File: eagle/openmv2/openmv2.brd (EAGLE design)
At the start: 43.2 x 54.6 mm, 82 parts, among them J3 CON_HEADER_1X03, J4 CON_HEADER_1X03, Q1 MOSFET, U1 TPS2114APW, U10 IS42S81600E-7TL, U2 USD-47571, U3 BEAD, U4 TPS768, U5 BEAD, U6 BEAD, U7 STM32F429, U8 VREG_25, U9 OV2640, X1 USB-MICROB

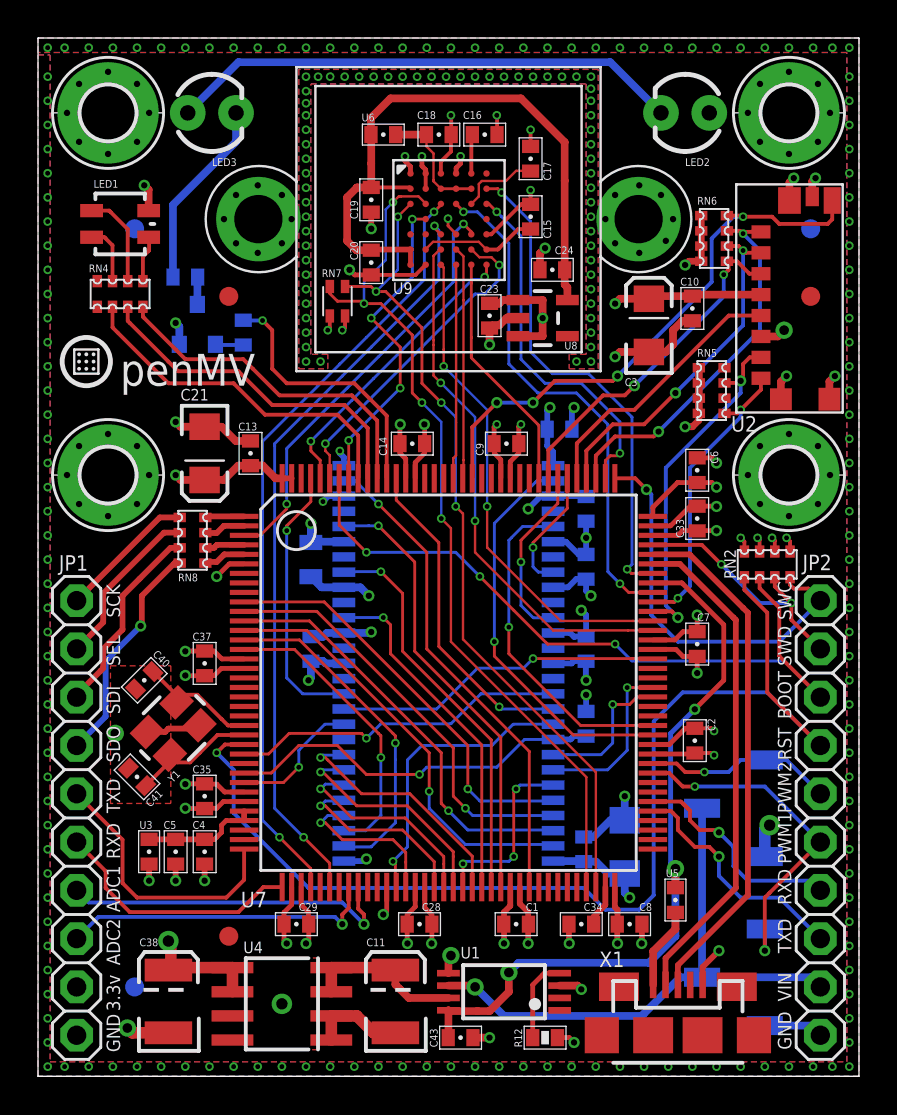
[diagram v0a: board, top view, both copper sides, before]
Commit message: Rename Eagle files
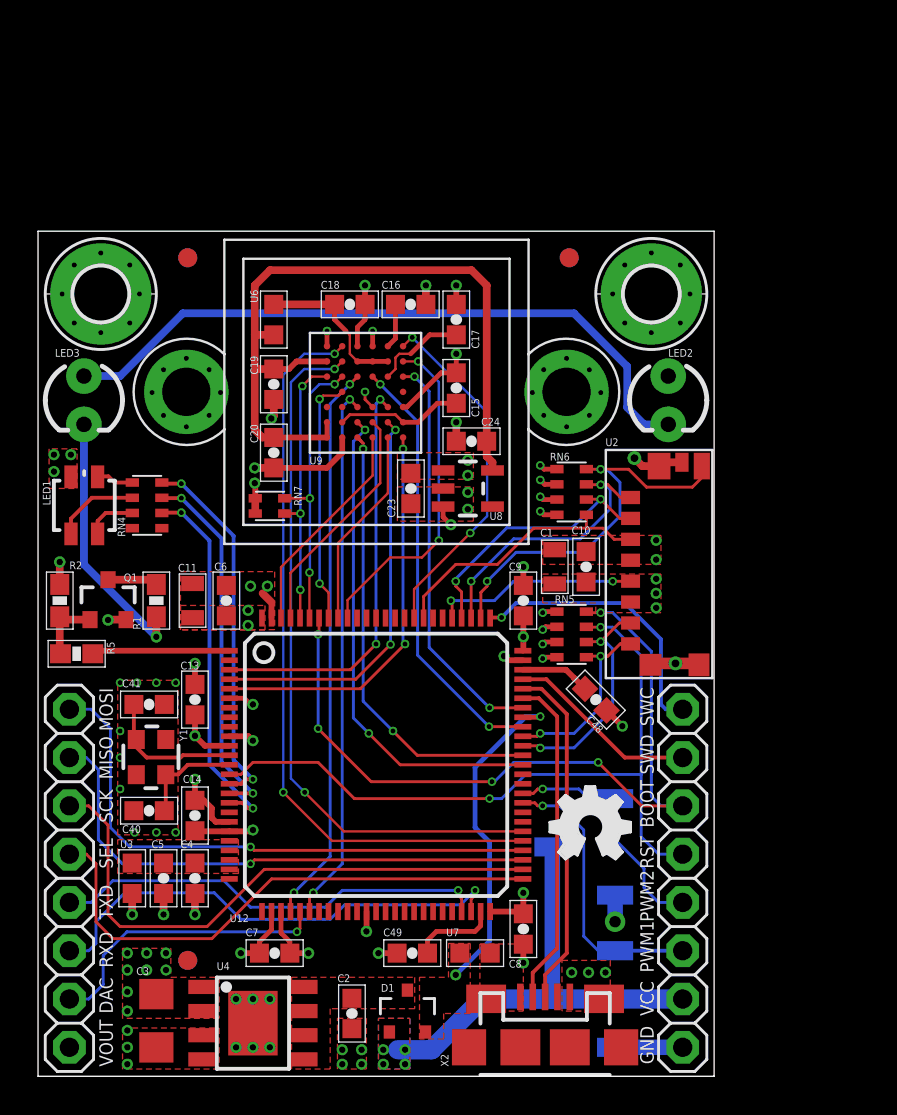
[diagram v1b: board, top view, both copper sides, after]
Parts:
- removed C12, C21: 100uF, sfe:EIA3216
- removed C25, C26, C27, C28, C29, C31, C32, C35, C36, C37, C43: 0.1uF, sfe:0402-CAP
- removed C30: 10uF, sfe:0805
- removed C33, C34: 2.2uF, sfe:0402-CAP
- removed C38: 100uF, sfe:EIA3528
- removed H1, H8: MOUNT-PAD-ROUND2.8, holes:2,8-PAD
- removed R12: 1K, sfe:0402-RES
- removed R4: 10ohm, iofault:0402-RES
- removed RN2, RN8: (no value), resistor-dil:CAT16
- removed U$1: LENSMOUNT, omnivision:LENSMOUNT
- removed U$14, U$15, U$16, U$17, U$19, U$20: FIDUCIAL, adafruit:FIDUCIAL_1MM
- removed U10: IS42S81600E-7TL, mux:TSOPII-54
- removed U5: BEAD, heka:0402-CAP
- removed X1: USB-MICROB, sfe:USB-MICROB
- added C48, C49: 2.2uF, sfe:0603-CAP
- added D1: BAT54C, diode:SOT23
- added JP3, JP4: (no value), pinhead:1X08
- added JP5, JP6, JP7, JP8: FIDUCIAL1X2, sfe:FIDUCIAL-1X2
- added R2: 10k, sfe:0603-RES
- added U$3: (no value), openmv:OMV-LOGO
- added U12: STM32F427-LQFP100, mux:LQFP100
- added X2: USB-MICROB, sfe:USB-MICROB
- C1: value 0.1uF -> 22uF; device sfe:0402-CAP -> sfe:0805
- C10, C13, C14, C15, C16, C17, C18, C19, C20, C4, C5, C6, C7, C8, C9: device sfe:0402-CAP -> sfe:0603-CAP
- C11: value 100uF -> 22uF; device sfe:EIA3528 -> sfe:0805
- C2: value 0.1uF -> 4.7uF; device sfe:0402-CAP -> sfe:0603-CAP
- C23, C24: value 10uF -> 4.7uF; device sfe:0402-CAP -> sfe:0603-CAP
- C3: device sfe:EIA3216 -> sfe:1206
- C40, C41: value 18pF -> 12pF; device sfe:0402-CAP -> sfe:0603-CAP
- JP1, JP2: value (none) -> FIDUCIAL1X2; device pinhead:1X10 -> sfe:FIDUCIAL-1X2
- LOGO1: value OSHW_LOGO_FILLX0200-NT -> OSHW_LOGO_FILLX0150-NT; device iofault:OSHW_FILLX200_NOTEXT -> iofault:OSHW_FILLX150_NOTEXT
- R1: value 10K -> 10ohm; device sfe:0402-RES -> sfe:0603-RES
- R5: device sfe:0402-RES -> sfe:0603-RES
- RN4: value (none) -> 220R; device resistor-dil:CAT16 -> resistor-dil:EXBV8V
- RN5, RN6: value (none) -> 10K; device resistor-dil:CAT16 -> resistor-dil:EXBV8V
- RN7: value (none) -> 10K
- U1: value TPS2114APW -> LENSMOUNT20MM; device mux:TSSOP8 -> omnivision:LENSMOUNT-20MM
- U3, U6: value BEAD -> (none); device heka:0402-CAP -> sfe:0603
- U4: value TPS768 -> BD33IA; device mux:SOIC8 -> mux:HTSOP-J8
- U7: value STM32F429 -> (none); device stm32:LQFP144 -> sfe:0603
- U8: value VREG_25 -> VREG_28
- Y1: device mux:CRYSTAL3.2X2.5 -> mux:CRYSTAL-2.5X2.0
- moved C3 44.8 mm to (6.22, 2.92), turned to 270 degrees
- moved H2 37.4 mm to (3.30, 41.1)
- moved JP2 34.1 mm to (7.87, 6.10), flipped to the bottom, turned to 0 degrees
- moved U1 32.3 mm to (17.8, 36.0), turned to 0 degrees
- moved H6 30.1 mm to (32.3, 41.1)
- moved C7 27.5 mm to (12.4, 6.48), turned to 180 degrees
- moved C6 25.7 mm to (9.91, 25.0)
- moved C11 23.6 mm to (8.13, 25.0), turned to 270 degrees
- moved R1 23.5 mm to (6.22, 25.0), flipped to the top
- moved C2 23.0 mm to (16.5, 3.30)
- moved C14 22.7 mm to (8.26, 13.7), turned to 270 degrees
- moved R5 19.0 mm to (2.03, 22.2), flipped to the top, turned to 180 degrees
- moved C1 18.9 mm to (27.2, 26.8), turned to 270 degrees
- moved LOGO1 16.7 mm to (26.9, 11.4), flipped to the top
- moved LED3 16.5 mm to (2.41, 35.6), turned to 270 degrees
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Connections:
- removed net ADC12_IN14: JP1.8, U7.44
- removed net ADC12_IN15: JP1.7, U7.45
- removed net ADC12_IN5: U7.41
- removed net DCMI_SCL: RN7.2, U7.69, U9.C2
- removed net DCMI_SDA: RN7.1, U7.70, U9.C1
- removed net DRAM_A0: U10.23, U7.10
- removed net DRAM_A1: U10.24, U7.11
- removed net DRAM_A10: U10.22, U7.56
- removed net DRAM_A11: U10.35, U7.57
- removed net DRAM_A2: U10.25, U7.12
- removed net DRAM_A3: U10.26, U7.13
- removed net DRAM_A4: U10.29, U7.14
- removed net DRAM_A5: U10.30, U7.15
- removed net DRAM_A6: U10.31, U7.50
- removed net DRAM_A7: U10.32, U7.53
- removed net DRAM_A8: U10.33, U7.54
- removed net DRAM_A9: U10.34, U7.55
- removed net DRAM_BA0: U10.20, U7.89
- removed net DRAM_BA1: U10.21, U7.90
- removed net DRAM_CAS: U10.17, U7.132
- removed net DRAM_CLK: U10.38, U7.93
- removed net DRAM_CLKE: U10.37, U7.29
- removed net DRAM_CS: R1.2, U10.19, U7.28
- removed net DRAM_D0: U10.2, U7.85
- removed net DRAM_D1: U10.5, U7.86
- removed net DRAM_D2: U10.8, U7.114
- removed net DRAM_D3: U10.11, U7.115
- removed net DRAM_D4: U10.44, U7.58
- removed net DRAM_D5: U10.47, U7.59
- removed net DRAM_D6: U10.50, U7.60
- removed net DRAM_D7: U10.53, U7.63
- removed net DRAM_DQM: U10.39, U7.141
- removed net DRAM_RAS: U10.18, U7.49
- removed net DRAM_WE: U10.16, U7.26
- removed net FS_DN: U7.103, X1.D-
- removed net N$15: U7.128
- removed net N$17: U7.92
- removed net N$18: U7.18
- removed net N$19: U7.91
- removed net N$20: JP1.1, RN8.1
- removed net N$21: JP1.2, RN8.2
- removed net N$22: U5.1, X1.VBUS
- removed net N$23: JP1.3, RN8.3
- removed net N$24: JP1.4, RN8.4
- removed net N$25: U7.122
- removed net N$26: R12.2, U1.4
- removed net N$27: U7.19
- removed net N$28: U7.20
- removed net SPI4_MISO: RN8.6, U7.4
- removed net SPI4_MOSI: RN8.5, U7.5
- removed net SPI4_NSS: RN8.7, U7.2
- removed net SPI4_SCK: RN8.8, U7.1
- removed net TIM12_CH1: U7.75
- removed net TIM12_CH2: U7.76
- removed net USART2_RX: JP1.6, U7.37
- removed net USART2_TX: JP1.5, U7.36
- removed net USART3_RX: JP2.7, U7.78
- removed net USART3_TX: JP2.8, U7.77
- removed net VBAT: J3.2, J4.2, JP2.9, U1.6
- new net DAC: JP4.7, U12.30
- new net EXPST: U12.55, U9.A2
- new net FREX: U12.56, U9.B2
- new net FS_DM: U12.70, X2.D-
- new net I2C1_SCL: RN7.2, U12.95, U9.C2
- new net I2C1_SDA: RN7.1, U12.96, U9.C1
- new net I2C2_SCL: JP4.5, U12.47
- new net I2C2_SDA: JP4.6, U12.48
- new net RAW: D1.1, J3.2, J4.2, JP3.7
- new net SPI2_MISO: JP4.2, U12.53
- new net SPI2_MOSI: JP4.1, U12.54
- new net SPI2_NSS: JP4.4, U12.51
- new net SPI2_SCLK: JP4.3, U12.52
- new net STROBE: U12.84, U9.A6
- net BOOT0: now also JP3.3, RN5.8, U12.94; no longer JP2.3, RN2.6, U7.138
- net DCMI_CLK: now also U12.67; no longer U7.100
- net DCMI_D0: now also U12.63; no longer U7.96
- net DCMI_D1: now also U12.64; no longer U7.97
- net DCMI_D2: now also U12.97; no longer U7.125
- net DCMI_D3: now also U12.98; no longer U7.126
- net DCMI_D4: now also U12.3; no longer U7.3
- net DCMI_D5: now also U12.92; no longer U7.117
- net DCMI_D6: now also U12.4; no longer U7.139
- net DCMI_D7: now also U12.5; no longer U7.140
- net DCMI_HSYNC: now also U12.29; no longer U7.40
- net DCMI_PCLK: now also U12.31; no longer U7.42
- net DCMI_PWDN: now also U12.91; no longer U7.102
- net DCMI_RST: now also U12.69; no longer U7.110
- net DCMI_VSYNC: now also U12.93; no longer U7.137
- net FS_DP: now also U12.71, X2.D+; no longer U7.104, X1.D+
- net GND: now also C11.1, C3.2, C48.2, C49.2, JP3.8, R2.1, RN5.1, U12.10, U12.20, U12.27, U12.37, U12.74, U12.99, U4.3, U4.P$1, X2.GND; no longer C11.C, C12.C, C21.C, C25.2, C26.2, C27.2, C28.1, C29.2, C3.C, C30.2, C31.2, C32.2, C33.2, C34.2, C35.2, C36.2, C37.2, C38.C, C43.2, H1.B2,8, H2.B2,8, H6.B2,8, H8.B2,8, JP1.10, JP2.10, R12.1, RN2.1, RN2.3, U$1.P$1, U$1.P$2, U1.3, U1.5, U10.12, U10.28, U10.41, U10.46, U10.52, U10.54, U10.6, U4.1, U4.2, U7.107, U7.120, U7.130, U7.16, U7.31, U7.38, U7.48, U7.51, U7.61, U7.83, U7.94, U9.A2, U9.B2, X1.GND
- net LED_B: now also U12.16; no longer U7.135
- net LED_G: now also U12.17; no longer U7.136
- net LED_IR: now also U12.1; no longer U7.133
- net LED_R: now also U12.15; no longer U7.134
- net N$10: now also R1.2; no longer R4.1
- net N$12: now also C4.1, C5.1, U12.21, U12.22, U3.1; no longer U7.127
- net N$14: now also R1.1; no longer R4.2
- net N$2: now also U12.13; no longer U7.23
- net N$4: now also U12.12; no longer U7.24
- net N$5: now also R2.2
- net N$7: now also U7.1, X2.VBUS; no longer C4.1, C5.1, U3.1, U7.32, U7.33
- net NRST: now also JP3.4, RN5.7, U12.14; no longer JP2.4, RN2.5, U7.25
- net SDIO_CLK: now also U12.80; no longer U7.113
- net SDIO_CMD: now also U12.83; no longer U7.116
- net SDIO_D0: now also RN5.6, U12.65; no longer RN5.7, U7.98
- net SDIO_D1: now also U12.66; no longer U7.99
- net SDIO_D2: now also U12.78; no longer U7.111
- net SDIO_D3: now also U12.79; no longer U7.112
- net SD_CD: now also U12.77; no longer U7.124
- net SWCLK: now also JP3.1, U12.76; no longer JP2.1, RN2.8, U7.109
- net SWDIO: now also JP3.2, U12.72; no longer JP2.2, RN2.7, U7.105
- net TIM4_CH1: now also JP3.6, U12.59; no longer JP2.6, U7.81
- net TIM4_CH2: now also JP3.5, U12.60; no longer JP2.5, U7.82
- net VBUS: now also D1.2, U12.68, U7.2; no longer C43.1, U1.8, U5.2, U7.101
- net VCAP1: now also C49.1, U12.49; no longer C34.1, U7.71
- net VCAP2: now also C48.1, U12.73; no longer C33.1, U7.106
- net VCC: now also C11.2, C3.1, JP4.8, U12.100, U12.11, U12.19, U12.28, U12.50, U12.6, U12.75, U4.1, U4.2; no longer C12.A, C2.1, C21.A, C25.1, C26.1, C27.1, C28.2, C29.1, C3.A, C30.1, C31.1, C32.1, C35.1, C36.1, C37.1, C38.A, JP1.9, R1.1, RN2.2, RN2.4, RN5.1, U10.1, U10.14, U10.27, U10.3, U10.43, U10.49, U10.9, U4.5, U4.6, U7.108, U7.121, U7.131, U7.143, U7.144, U7.17, U7.30, U7.39, U7.52, U7.6, U7.62, U7.72, U7.84, U7.95
- net VIN: now also C2.1, D1.3, U4.5, U4.8; no longer C11.A, U1.7, U4.3, U4.4
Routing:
- net VCC: track 102.3 -> 26.3 mm, vias 32 -> 33
- net GND: track 123.5 -> 53.8 mm, vias 319 -> 61
- net DCMI_SCL: track 46.4 -> 0.00 mm, vias 4 -> 0
- net DCMI_SDA: track 43.5 -> 0.00 mm, vias 4 -> 0
- net EXPST: track 0.00 -> 39.3 mm, vias 0 -> 2
- net FREX: track 0.00 -> 37.3 mm, vias 0 -> 2
- net SPI2_SCLK: track 0.00 -> 30.5 mm
- net VBAT: track 30.2 -> 0.00 mm, vias 1 -> 0
- net SPI2_MOSI: track 0.00 -> 30.0 mm, vias 0 -> 1
- net SPI2_NSS: track 0.00 -> 28.8 mm
- net SPI2_MISO: track 0.00 -> 28.4 mm, vias 0 -> 1
- net FS_DN: track 26.3 -> 0.00 mm
- net DRAM_D7: track 25.8 -> 0.00 mm, vias 1 -> 0
- net I2C2_SDA: track 0.00 -> 25.7 mm, vias 0 -> 1
- net RAW: track 0.00 -> 24.1 mm, vias 0 -> 4
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- added copper zone on layer 1, net N$12
- added copper zone on layer 1, net N$7
- added copper zone on layer 1, net RAW
- added copper zone on layer 16, net RAW
- added copper zone on layer 1, net VBUS
- added copper zone on layer 1, net VCC
- added copper zone on layer 1, net VIN
- removed copper zone on layer 16, net GND
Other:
- board size 43.2 x 54.6 mm -> 35.6 x 44.5 mm
- board text added: "DAC"
- board text added: "MISO"
- board text added: "MOSI"
- board text added: "VCC"
- board text added: "VOUT"
- board text removed: "3.3v"
- board text removed: "ADC1"
- board text removed: "ADC2"
- board text removed: "OpenMV2 R1"
- board text removed: "SDI"
- board text removed: "SDO"
- board text removed: "VIN"
- board text removed: "penMV"
